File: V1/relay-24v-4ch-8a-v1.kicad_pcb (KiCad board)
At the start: 2 copper layers, 53 x 67.8 mm, 24 parts, among them J1 DB141V-2.54-2P, J2 DB141V-2.54-4P, J3 DB142V-5.08-4P, J4 DB142V-5.08-4P, K1 G5Q-1A4-DC24V, K2 G5Q-1A4-DC24V, K3 G5Q-1A4-DC24V, K4 G5Q-1A4-DC24V

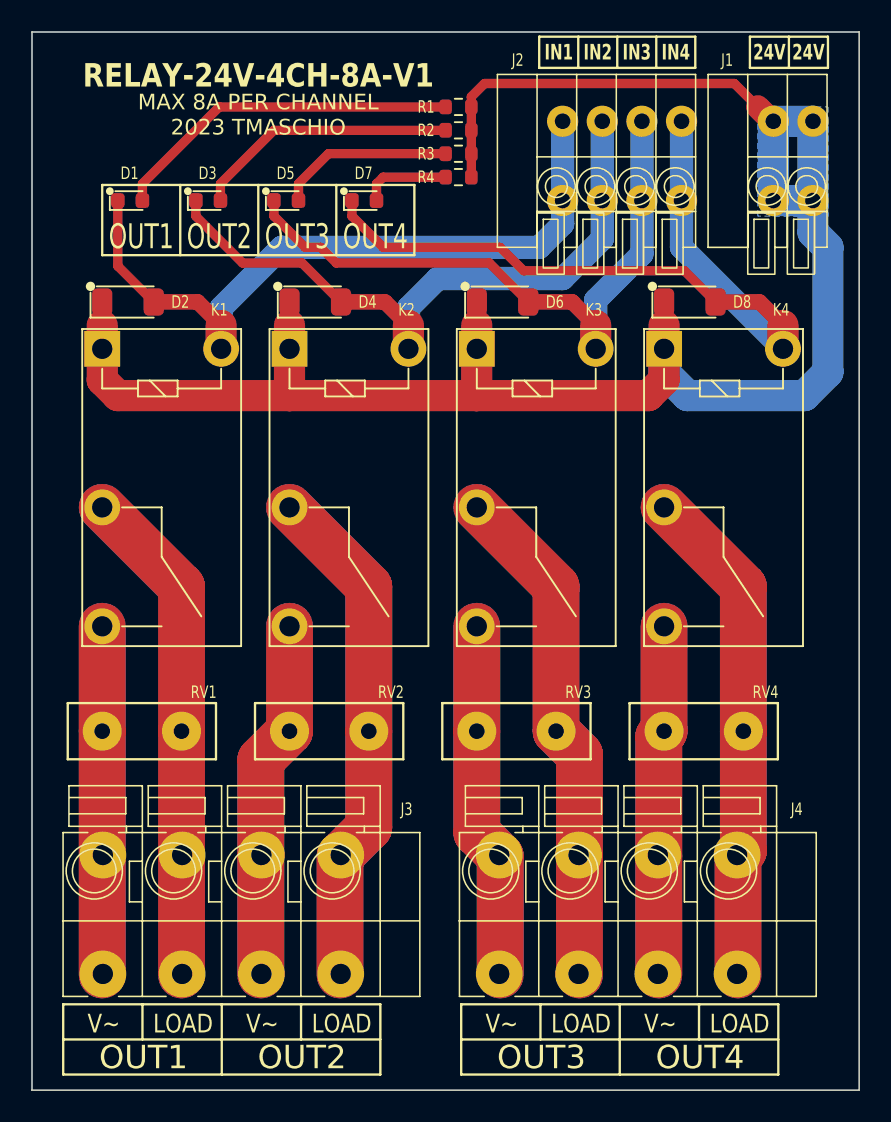
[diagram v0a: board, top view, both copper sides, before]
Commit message: Revising for fabrication
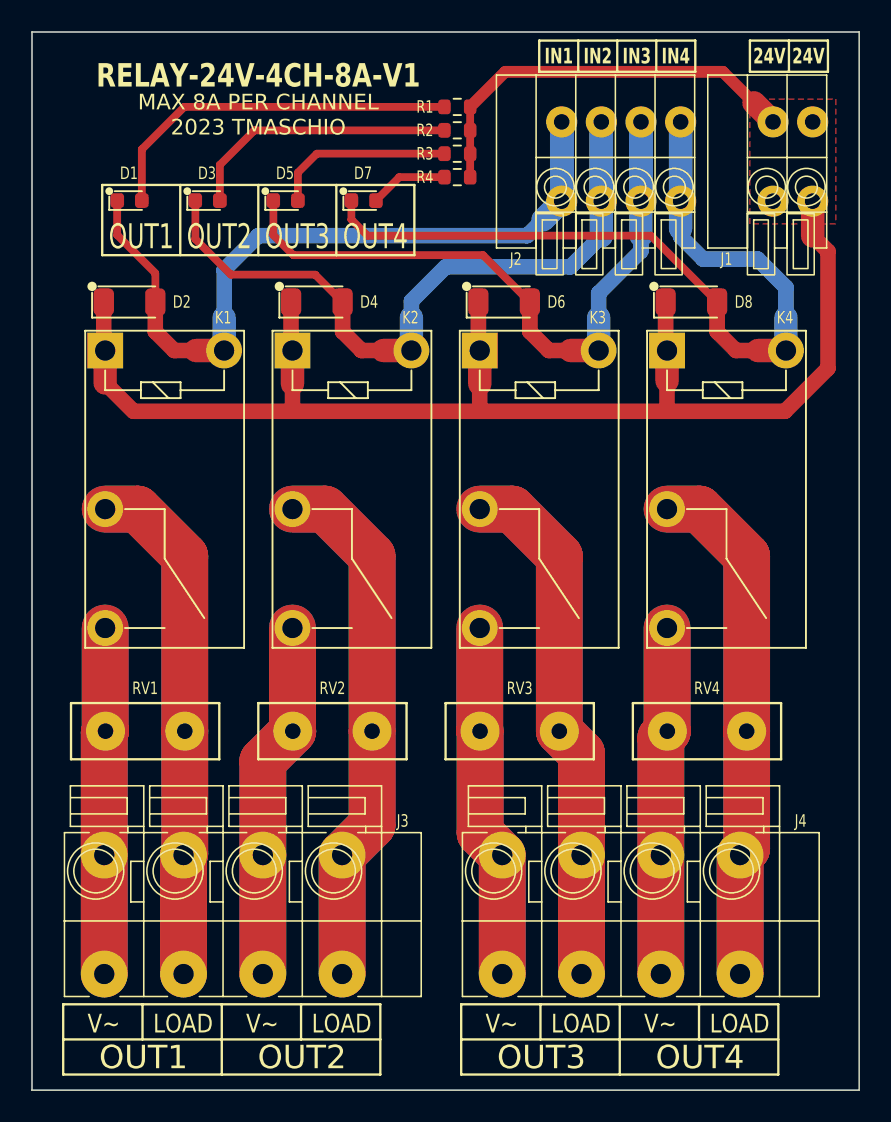
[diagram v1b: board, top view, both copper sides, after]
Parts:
- D1, D3, D5, D7: value EMERALD -> WHITE
- R1, R2, R3, R4: value 6k8/100mW -> 10k/100mW
- moved K1 9.85 mm to (133.5, 91.5)
- moved K2 9.85 mm to (145.5, 91.5)
- moved K3 9.85 mm to (157.5, 91.5)
- moved K4 9.85 mm to (169.5, 91.5)
- moved J4 8.69 mm to (162.8, 118.8)
- moved J3 8.60 mm to (137.2, 118.8)
- moved J2 4.65 mm to (162.8, 70.5)
- moved J1 2.88 mm to (173.8, 70.5)
- moved RV1 2.75 mm to (132.2, 107.0)
- moved RV2 2.75 mm to (144.2, 107.0)
- moved RV3 2.75 mm to (156.2, 107.0)
- moved RV4 2.75 mm to (168.2, 107.0)
- moved D2 0.10 mm to (131.2, 79.5)
- moved D4 0.10 mm to (143.2, 79.5)
- moved D6 0.10 mm to (155.2, 79.5)
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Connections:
- net Net-(D1-A) renamed /LED1
- net Net-(D1-K) renamed /IN1
- net Net-(D3-A) renamed /LED2
- net Net-(D3-K) renamed /IN2
- net Net-(D5-A) renamed /LED3
- net Net-(D5-K) renamed /IN3
- net Net-(D7-A) renamed /LED4
- net Net-(D7-K) renamed /IN4
- net Net-(J3-Pin_1) renamed /OUT1PW
- net Net-(J3-Pin_2) renamed /OUT1LD
- net Net-(J3-Pin_3) renamed /OUT2PW
- net Net-(J3-Pin_4) renamed /OUT2LD
- net Net-(J4-Pin_1) renamed /OUT3PW
- net Net-(J4-Pin_2) renamed /OUT3LD
- net Net-(J4-Pin_3) renamed /OUT4PW
- net Net-(J4-Pin_4) renamed /OUT4LD
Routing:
- net +24V: track 124.6 -> 111.8 mm
- net /IN4: track 50.3 -> 58.2 mm
- net /IN2: track 43.4 -> 49.8 mm
- net /IN3: track 41.8 -> 48.1 mm
- net /IN1: track 47.2 -> 53.1 mm
- net /OUT4LD: track 64.4 -> 66.6 mm
- net /OUT2LD: track 65.7 -> 67.8 mm
- net /OUT1LD: track 64.1 -> 66.3 mm
- net /OUT3LD: track 65.4 -> 67.4 mm
- net /LED1: track 22.5 -> 23.8 mm
- net /LED2: track 16.9 -> 17.6 mm
- net /LED4: track 5.68 -> 5.01 mm
- added copper zone on F.Cu, net +24V
- removed copper zone on B.Cu, net +24V
